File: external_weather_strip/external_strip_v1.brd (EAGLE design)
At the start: 35.2 x 15.2 mm, 12 parts, among them U2 SHT21, U3 ML8511-UV-SENSORSMD, U9 BMP180

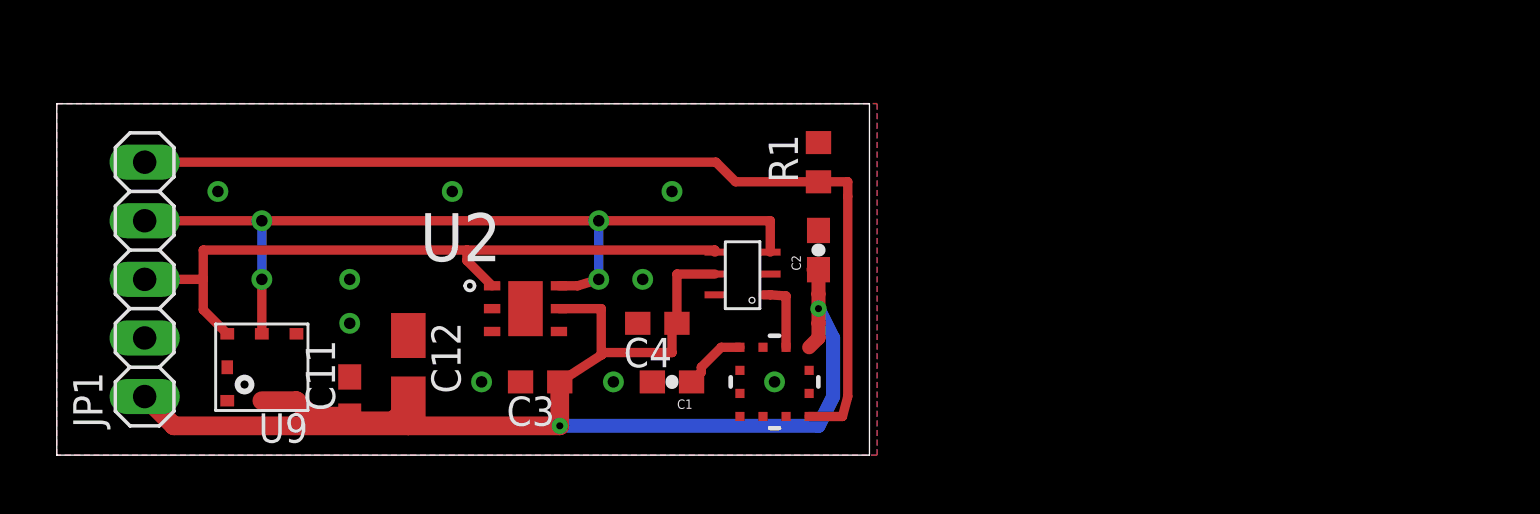
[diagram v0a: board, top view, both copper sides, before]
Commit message: finished weather strip
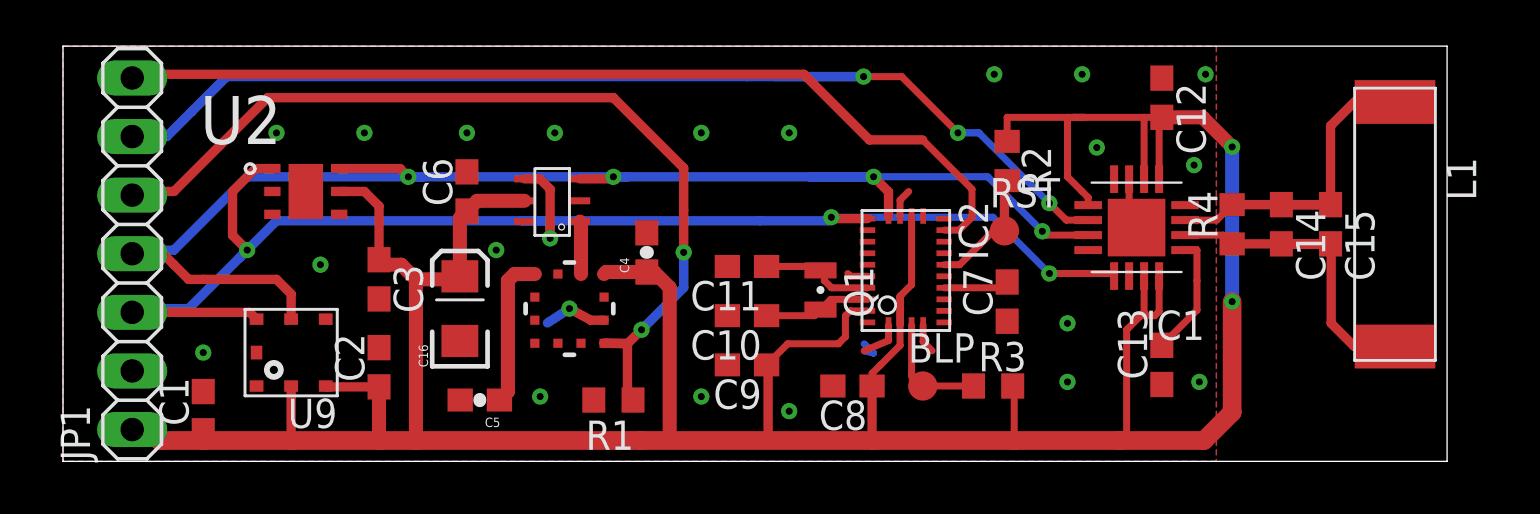
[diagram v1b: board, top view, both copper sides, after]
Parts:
- added BLP, RST: PTR1B1,27, testpad:B1,27
- added C10: 12p, rcl:C0603
- added C13: 10u, rcl:C0603
- added C14: 670p, rcl:C0603
- added C15: 270p, rcl:C0603
- added C16: 10uF, SparkFun-Retired:EIA3216
- added C5: 1n, SparkFun-Capacitors:0603-CAP
- added C6, C7, C8: 100n, rcl:C0603
- added C9: 120n, rcl:C0603
- added IC1: AS3935, AS3935:16LDMLPQ
- added IC2: BNO055A, BNO055:BNO055
- added L1: 100uH, AS3935:COILCRAFT
- added Q1: 32.768kHz, crystal:FC-12M
- added R2, R3: 10k, rcl:R0603
- added R4: 10k, resistor:R0603
- C1: value 1nF -> 100n; device SparkFun-Capacitors:0603-CAP -> rcl:C0603
- C11: value 100n -> 12p
- C12: value 10u -> 1u; device resistor:A/3216-18R -> rcl:C0603
- C2: value 0.1uF -> 100n; device SparkFun-Capacitors:0603-CAP -> rcl:C0603
- C4: device rcl:C0603 -> SparkFun-Capacitors:0603-CAP
- JP1: device Headerlibrary:1X05 -> pinhead:1X07
- moved C12 34.7 mm to (46.6, 16.8)
- moved C1 20.4 mm to (5.08, 3.17), turned to 90 degrees
- moved C2 19.7 mm to (12.7, 5.08)
- moved C11 18.1 mm to (28.7, 9.45), turned to 180 degrees
- moved R1 13.6 mm to (22.9, 3.66), turned to 180 degrees
- moved U2 10.8 mm to (9.53, 12.7)
- moved U3 9.44 mm to (21.0, 7.62)
- moved U$5 8.84 mm to (21.0, 10.8)
- moved C3 8.28 mm to (12.7, 8.89), turned to 270 degrees
- moved C4 3.11 mm to (24.3, 10.1), turned to 90 degrees
- moved U9 1.42 mm to (8.89, 5.71)
- moved JP1 1.23 mm to (2.00, 10.0)
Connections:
- new net ACCEL_IRQ: IC2.14, JP1.7
- new net ACCEL_N_BOOTLD: BLP.TP, IC2.4, R3.1
- new net ACCEL_N_RST: IC2.11, R2.2, RST.TP
- new net LIGHTNING_IRQ: IC1.10, JP1.6
- new net N$18: C7.2, IC2.9
- new net N$19: C10.1, IC2.27, Q1.2
- new net N$2: C13.2, IC1.1
- new net N$5: C14.1, C15.1, IC1.3, L1.1, R4.2
- new net N$73: C11.1, IC2.26, Q1.1
- net +3V3: now also C1.1, C12.2, C16.A, C6.1, C8.1, C9.1, IC1.15, IC1.16, IC1.5, IC1.6, IC1.9, IC2.17, IC2.28, IC2.3, R2.1, R3.2; no longer C11.1, C12.+
- net GND: now also C10.2, C12.1, C13.1, C14.2, C15.2, C16.C, C5.2, C6.2, C7.1, C8.2, C9.2, IC1.2, IC1.4, IC1.7, IC1.EXP, IC2.10, IC2.15, IC2.16, IC2.18, IC2.2, IC2.25, IC2.5, IC2.6, L1.2, R4.1; no longer C12.-
- net N$3: now also C5.1; no longer C1.1
- net SCL: now also IC1.11, IC2.19
- net SDA: now also IC1.13, IC2.20
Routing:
- net +3V3: track 64.6 -> 173.3 mm
- net LIGHTNING_IRQ: track 0.00 -> 54.0 mm, vias 0 -> 3
- net ACCEL_IRQ: track 0.00 -> 41.2 mm
- net SDA: track 30.9 -> 63.1 mm, vias 0 -> 4
- net GND: track 0.00 -> 26.5 mm, vias 9 -> 21
- net SCL: track 37.7 -> 63.4 mm
- net N$5: track 0.00 -> 15.8 mm
- net ACCEL_N_RST: track 0.00 -> 5.45 mm
- net N$2: track 0.00 -> 5.28 mm
- net ACCEL_N_BOOTLD: track 0.00 -> 5.04 mm
- net N$73: track 0.00 -> 4.92 mm
- net N$19: track 0.00 -> 4.67 mm
- net N$3: track 2.84 -> 6.62 mm
- net N$18: track 0.00 -> 2.98 mm
- net UV_EN: track 42.5 -> 40.2 mm, vias 0 -> 2
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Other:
- board size 35.2 x 15.2 mm -> 60 x 18 mm
